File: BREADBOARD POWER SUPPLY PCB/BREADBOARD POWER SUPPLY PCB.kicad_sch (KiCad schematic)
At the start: 17 parts, among them J1 Conn_01x02_Pin, J2 Conn_01x02_Pin, J3 Conn_01x03_Pin, J4 Conn_01x03_Pin, J5 Screw_Terminal_01x02, J6 Barrel_Jack_Switch, J7 Screw_Terminal_01x02, U1 LM7805_TO220, U2 LM317_TO-220

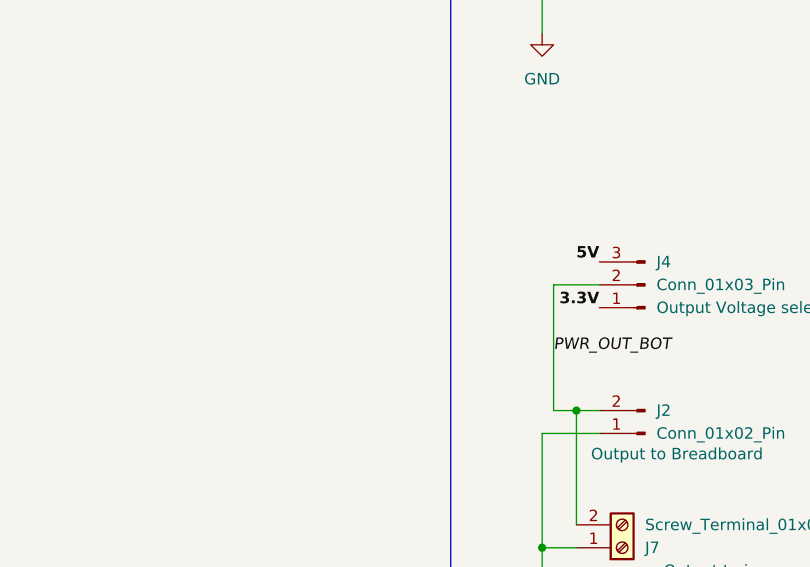
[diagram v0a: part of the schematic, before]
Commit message: Added a capacitor and updated gitignore.
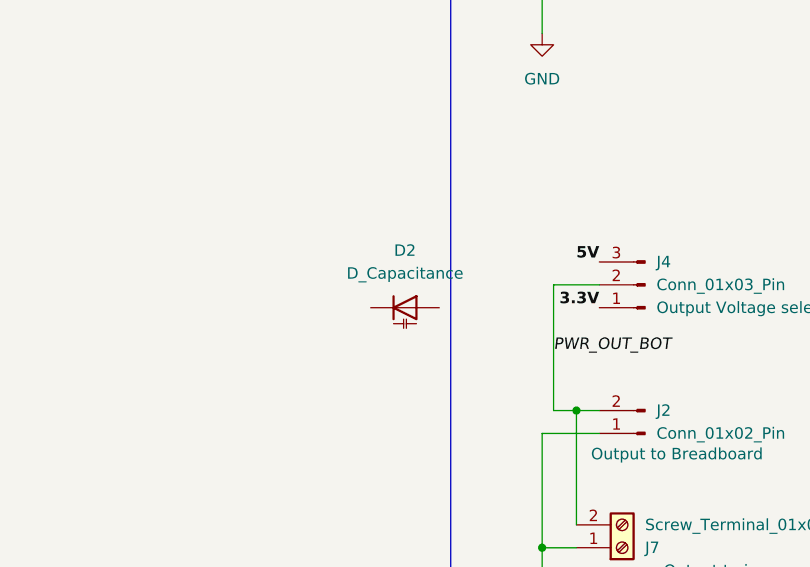
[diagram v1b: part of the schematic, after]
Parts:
- added D2: D_Capacitance, symbol Device:D_Capacitance
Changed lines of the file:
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@@
+	)
+	(symbol
+		(lib_id "Device:D_Capacitance")
+		(at 165.1 111.76 0)
+		(unit 1)
+		(exclude_from_sim no)
+		(in_bom yes)
+		(on_board yes)
+		(dnp no)
+		(fields_autoplaced yes)
+		(property "Reference" "D2"
+			(at 165.1 105.41 0)
+			(effects
+				(font
+					(size 1.27 1.27)
+				)
+			)
+		)
+		(property "Value" "D_Capacitance"
+			(at 165.1 107.95 0)
+			(effects
+				(font
+					(size 1.27 1.27)
+				)
+			)
+		)
+		(property "Footprint" ""
+			(at 165.1 111.76 0)
+			(effects
+				(font
+					(size 1.27 1.27)
+				)
+				(hide yes)
+			)
+		)
+		(property "Datasheet" "~"
+			(at 165.1 111.76 0)
+			(effects
+				(font
+					(size 1.27 1.27)
+				)
+				(hide yes)
+			)
+		)
+		(property "Description" "Variable capacitance diode"
+			(at 165.1 111.76 0)
+			(effects
+				(font
+					(size 1.27 1.27)
+				)
+				(hide yes)
+			)
+		)
+		(pin "2"
+		)
+		(pin "1"
+		)
+		(instances
+			(project "BREADBOARD POWER SUPPLY PCB"
+				(path "/1cd576f6-8893-4044-964a-3f3f3764ddce"
+					(reference "D2")
+					(unit 1)
+				)
+			)
+		)
 	)
 	(symbol

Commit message: Deleted the capcitnce from main branch.
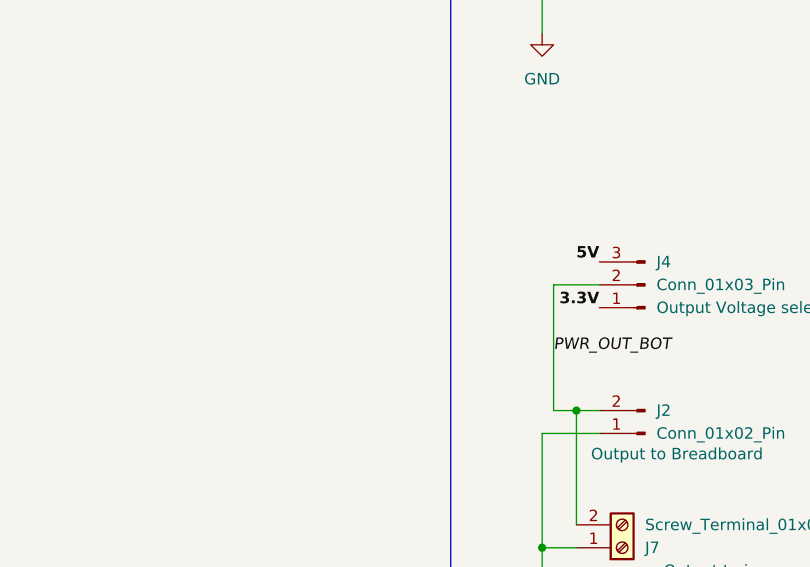
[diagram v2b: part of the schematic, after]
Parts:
- removed D2: D_Capacitance, symbol Device:D_Capacitance
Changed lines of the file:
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@@
-	)
-	(symbol
-		(lib_id "Device:D_Capacitance")
-		(at 165.1 111.76 0)
-		(unit 1)
-		(exclude_from_sim no)
-		(in_bom yes)
-		(on_board yes)
-		(dnp no)
-		(fields_autoplaced yes)
-		(property "Reference" "D2"
-			(at 165.1 105.41 0)
-			(effects
-				(font
-					(size 1.27 1.27)
-				)
-			)
-		)
-		(property "Value" "D_Capacitance"
-			(at 165.1 107.95 0)
-			(effects
-				(font
-					(size 1.27 1.27)
-				)
-			)
-		)
-		(property "Footprint" ""
-			(at 165.1 111.76 0)
-			(effects
-				(font
-					(size 1.27 1.27)
-				)
-				(hide yes)
-			)
-		)
-		(property "Datasheet" "~"
-			(at 165.1 111.76 0)
-			(effects
-				(font
-					(size 1.27 1.27)
-				)
-				(hide yes)
-			)
-		)
-		(property "Description" "Variable capacitance diode"
-			(at 165.1 111.76 0)
-			(effects
-				(font
-					(size 1.27 1.27)
-				)
-				(hide yes)
-			)
-		)
-		(pin "2"
-		)
-		(pin "1"
-		)
-		(instances
-			(project "BREADBOARD POWER SUPPLY PCB"
-				(path "/1cd576f6-8893-4044-964a-3f3f3764ddce"
-					(reference "D2")
-					(unit 1)
-				)
-			)
-		)
 	)
 	(symbol
